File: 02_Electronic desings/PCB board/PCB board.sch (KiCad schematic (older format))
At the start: 26 parts, among them J1 M1 Encoder, J10 Switch Manual/Auto, J11 Jetson, J12 Compass, J14 Arduino_Header, J15 M2_Controll, J16 Power +5V, J17 GPS, J18 Power +5V, J19 Power +5V, J2 M2 Encoder, J20 I2C, J21 Power +5V, J22 XBee, J3 Power +5V, J4 M1 encoder, J5 PS2_Controll, J6 M2 encoder, J8 Arduino_Mega_Header, J9 M1_Controll, M1 Hercules_motordriver, M2 Hercules_motordriver, U1 PS2_Receiver, U2 BNO055, U3 Logic_Level_Converter, U4 Screw_term_p2_5mm

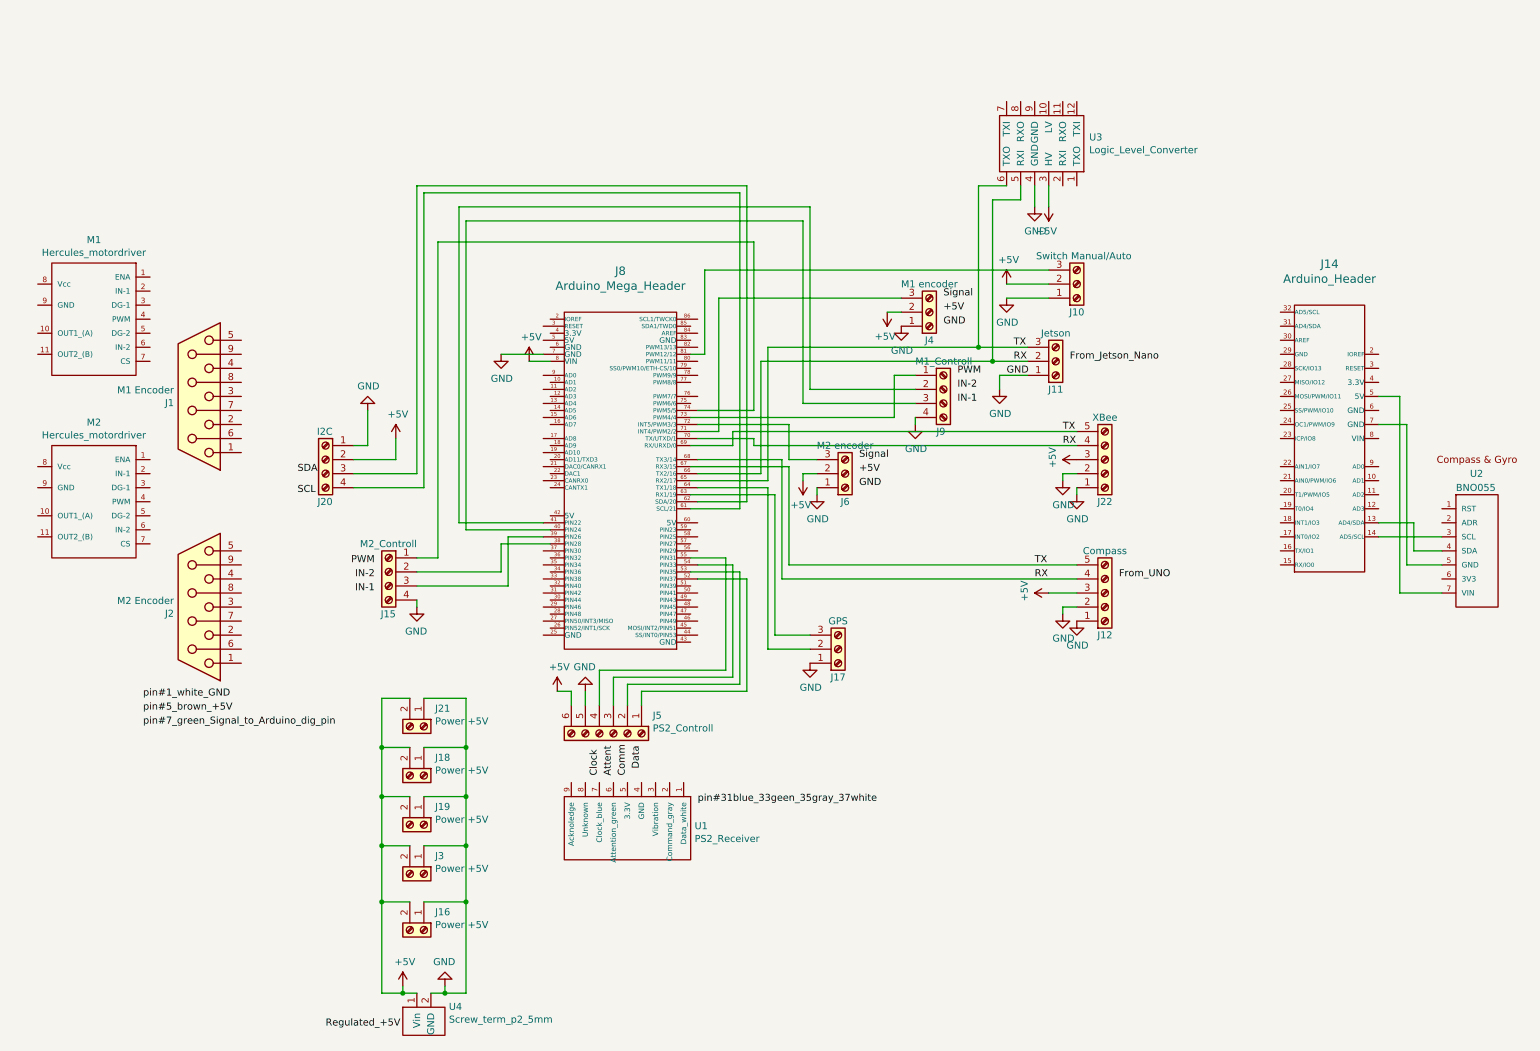
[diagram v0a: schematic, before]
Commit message: Upade
new version
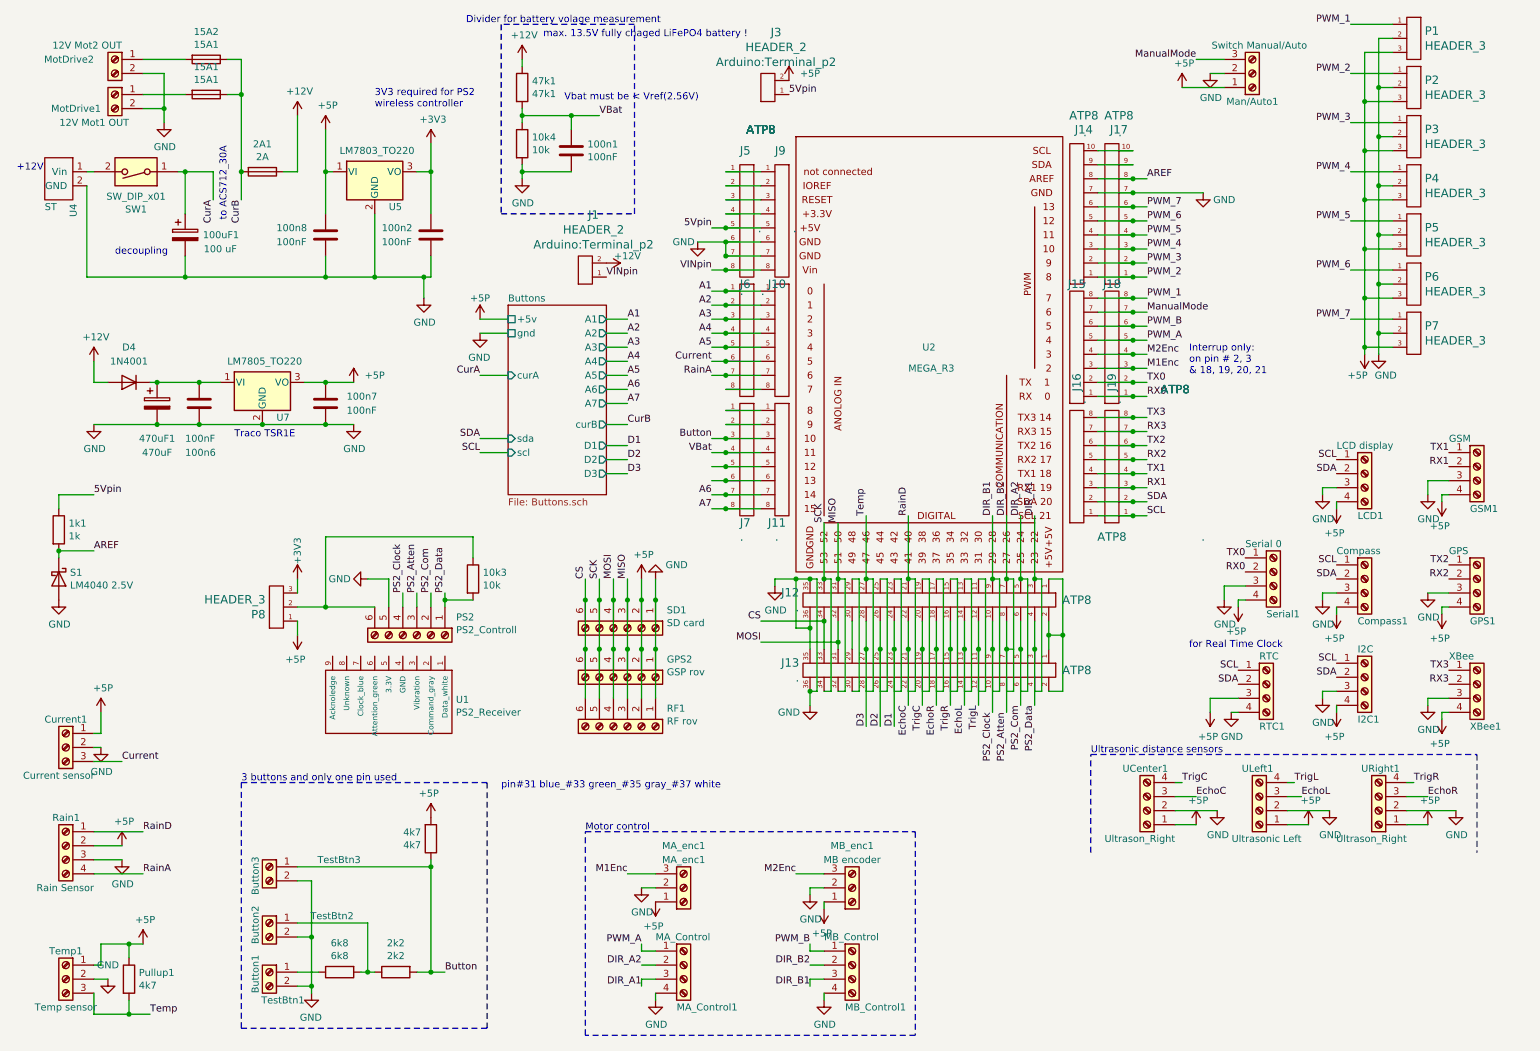
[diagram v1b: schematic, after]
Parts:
- removed J1: M1 Encoder, symbol Connector:DB9_Female
- removed J11: Jetson, TerminalBlock_TE-Connectivity:TerminalBlock_TE_282834-3_1x03_P2.54mm_Horizontal, symbol Connector:Screw_Terminal_01x03
- removed J12: Compass, TerminalBlock_TE-Connectivity:TerminalBlock_TE_282834-5_1x05_P2.54mm_Horizontal, symbol Connector:Screw_Terminal_01x05
- removed J14: Arduino_Header, symbol w_connectors:Arduino_Header
- removed J15: M2_Controll, TerminalBlock_TE-Connectivity:TerminalBlock_TE_282834-4_1x04_P2.54mm_Horizontal, symbol Connector:Screw_Terminal_01x04
- removed J16, J18, J19, J21, J3: Power +5V, TerminalBlock_TE-Connectivity:TerminalBlock_TE_282834-2_1x02_P2.54mm_Horizontal, symbol Connector:Screw_Terminal_01x02
- removed J17: GPS, TerminalBlock_TE-Connectivity:TerminalBlock_TE_282834-3_1x03_P2.54mm_Horizontal, symbol Connector:Screw_Terminal_01x03
- removed J2: M2 Encoder, symbol Connector:DB9_Female
- removed J20: I2C, TerminalBlock_TE-Connectivity:TerminalBlock_TE_282834-4_1x04_P2.54mm_Horizontal, symbol Connector:Screw_Terminal_01x04
- removed J22: XBee, TerminalBlock_TE-Connectivity:TerminalBlock_TE_282834-5_1x05_P2.54mm_Horizontal, symbol Connector:Screw_Terminal_01x05
- removed J8: Arduino_Mega_Header, Arduino:Arduino_MEGA, symbol w_connectors:Arduino_Mega_Header
- removed M1, M2: Hercules_motordriver, symbol My_symbol_library:Hercules_motordriver
- removed U2: BNO055, symbol My_symbol_library:BNO055
- removed U3: Logic_Level_Converter, Arduino:Logic_Level_Converter, symbol My_symbol_library:Logic_Level_Converter
- added 100n1, 100n2, 100n6, 100n7, 100n8: 100nF, Capacitor_THT:C_Disc_D10.5mm_W5.0mm_P5.00mm, symbol Device:C
- added 100uF1: 100 uF, Capacitor_THT:C_Radial_D8.0mm_H7.0mm_P3.50mm, symbol Device:CP
- added 10k3: 10k, Resistor_THT:R_Axial_DIN0207_L6.3mm_D2.5mm_P10.16mm_Horizontal, symbol Device:R
- added 10k4: 10k, Resistor_THT:R_Axial_DIN0309_L9.0mm_D3.2mm_P5.08mm_Vertical, symbol Device:R
- added 15A1, 15A2: 15A1, Shield:Fuse, symbol Device:Fuse
- added 1k1: 1k, Resistor_THT:R_Axial_DIN0207_L6.3mm_D2.5mm_P10.16mm_Horizontal, symbol Device:R
- added 2A1: 2A, Shield:Fuse, symbol Device:Fuse
- added 2k2: 2k2, Resistor_THT:R_Axial_DIN0309_L9.0mm_D3.2mm_P5.08mm_Vertical, symbol Device:R
- added 470uF1: 470uF, Capacitor_THT:C_Radial_D8.0mm_H7.0mm_P3.50mm, symbol Device:CP
- added 47k1: 47k1, Resistor_THT:R_Axial_DIN0309_L9.0mm_D3.2mm_P12.70mm_Horizontal, symbol Device:R
- added 4k7: 4k7, Resistor_THT:R_Axial_DIN0309_L9.0mm_D3.2mm_P5.08mm_Vertical, symbol Device:R
- added 6k8: 6k8, Resistor_THT:R_Axial_DIN0309_L9.0mm_D3.2mm_P5.08mm_Vertical, symbol Device:R
- added Button1: TestBtn1, Connector_JST:JST_XH_B2B-XH-A_1x02_P2.50mm_Vertical, symbol Connector:Screw_Terminal_01x02
- added Button2: TestBtn2, Connector_JST:JST_XH_B2B-XH-A_1x02_P2.50mm_Vertical, symbol Connector:Screw_Terminal_01x02
- added Button3: TestBtn3, Connector_JST:JST_XH_B2B-XH-A_1x02_P2.50mm_Vertical, symbol Connector:Screw_Terminal_01x02
- added Compass1: Compass, Connector_JST:JST_XH_B4B-XH-A_1x04_P2.50mm_Vertical, symbol Connector:Screw_Terminal_01x04
- added Current1: Current sensor, Connector_JST:JST_XH_B3B-XH-A_1x03_P2.50mm_Vertical, symbol Connector:Screw_Terminal_01x03
- added D4: 1N4001, Diode_THT:D_5W_P5.08mm_Vertical_AnodeUp, symbol Simulation_SPICE:DIODE
- added GPS1: GPS, Connector_JST:JST_XH_B4B-XH-A_1x04_P2.50mm_Vertical, symbol Connector:Screw_Terminal_01x04
- added GPS2: GSP rov, Connector_JST:JST_XH_B6B-XH-A_1x06_P2.50mm_Vertical, symbol Connector:Screw_Terminal_01x06
- added GSM1: GSM, Connector_JST:JST_XH_B4B-XH-A_1x04_P2.50mm_Vertical, symbol Connector:Screw_Terminal_01x04
- added I2C1: I2C, Connector_JST:JST_XH_B4B-XH-A_1x04_P2.50mm_Vertical, symbol Connector:Screw_Terminal_01x04
- added J1, J3: HEADER_2, Arduino:Terminal_p2, symbol w_connectors:HEADER_2
- added J10, J11, J15, J18, J19, J5, J6, J7, J9: ., ATP8, symbol w_connectors:HEADER_8
- added J12, J13: ., ATP8, symbol w_connectors:HEADER_18x2
- added J14, J17: ., ATP8, symbol w_connectors:HEADER_10
- added J16: ., ., symbol w_connectors:HEADER_8
- added LCD1: LCD display, Connector_JST:JST_XH_B4B-XH-A_1x04_P2.50mm_Vertical, symbol Connector:Screw_Terminal_01x04
- added MB_Control1: MB_Control, Connector_JST:JST_XH_B4B-XH-A_1x04_P2.50mm_Vertical, symbol Connector:Screw_Terminal_01x04
- added MotDrive1: 12V Mot1 OUT, TerminalBlock_Phoenix:TerminalBlock_Phoenix_MKDS-1,5-2-5.08_1x02_P5.08mm_Horizontal, symbol Connector:Screw_Terminal_01x02
- added MotDrive2: 12V Mot2 OUT, TerminalBlock_Phoenix:TerminalBlock_Phoenix_MKDS-1,5-2-5.08_1x02_P5.08mm_Horizontal, symbol Connector:Screw_Terminal_01x02
- added P1, P2, P3, P4, P5, P6, P7: HEADER_3, Arduino:Terminal_p3_sp, symbol w_connectors:HEADER_3
- added P8: HEADER_3, Arduino:Terminal_p3, symbol w_connectors:HEADER_3
- added Pullup1: 4k7, Resistor_THT:R_Axial_DIN0207_L6.3mm_D2.5mm_P10.16mm_Horizontal, symbol Device:R
- added RF1: RF rov, Connector_JST:JST_XH_B6B-XH-A_1x06_P2.50mm_Vertical, symbol Connector:Screw_Terminal_01x06
- added RTC1: RTC, Connector_JST:JST_XH_B4B-XH-A_1x04_P2.50mm_Vertical, symbol Connector:Screw_Terminal_01x04
- added Rain1: Rain Sensor, Connector_JST:JST_XH_B4B-XH-A_1x04_P2.50mm_Vertical, symbol Connector:Screw_Terminal_01x04
- added S1: LM4040 2.5V, Arduino:TO-92, symbol Device:D_Schottky
- added SD1: SD card, Connector_JST:JST_XH_B6B-XH-A_1x06_P2.50mm_Vertical, symbol Connector:Screw_Terminal_01x06
- added SW1: SW_DIP_x01, TerminalBlock_Phoenix:TerminalBlock_Phoenix_MKDS-1,5-2-5.08_1x02_P5.08mm_Horizontal, symbol Switch:SW_DIP_x01
- added Serial1: Serial 0, Connector_JST:JST_XH_B4B-XH-A_1x04_P2.50mm_Vertical, symbol Connector:Screw_Terminal_01x04
- added Temp1: Temp sensor, Connector_JST:JST_XH_B3B-XH-A_1x03_P2.50mm_Vertical, symbol Connector:Screw_Terminal_01x03
- added U2: MEGA_R3, symbol My_symbol_library:MEGA_R3
- added U5: LM7803_TO220, Package_TO_SOT_THT:TO-220-3_Vertical, symbol Regulator_Linear:LM7805_TO220
- added U7: LM7805_TO220, My_footprint_library:Traco_TSR2, symbol Regulator_Linear:LM7805_TO220
- added UCenter1, URight1: Ultrason_Right, Connector_JST:JST_XH_B4B-XH-A_1x04_P2.50mm_Vertical, symbol Connector:Screw_Terminal_01x04
- added ULeft1: Ultrasonic Left, Connector_JST:JST_XH_B4B-XH-A_1x04_P2.50mm_Vertical, symbol Connector:Screw_Terminal_01x04
- added XBee1: XBee, Connector_JST:JST_XH_B4B-XH-A_1x04_P2.50mm_Vertical, symbol Connector:Screw_Terminal_01x04
- MA_Control1: renamed from J9; value M1_Controll -> MA_Control; footprint TerminalBlock_TE-Connectivity:TerminalBlock_TE_282834-4_1x04_P2.54mm_Horizontal -> Connector_JST:JST_XH_B4B-XH-A_1x04_P2.50mm_Vertical
- MA_enc1: renamed from J4; value M1 encoder -> MA_enc1; footprint TerminalBlock_TE-Connectivity:TerminalBlock_TE_282834-3_1x03_P2.54mm_Horizontal -> Connector_JST:JST_XH_B3B-XH-A_1x03_P2.50mm_Vertical
- MB_enc1: renamed from J6; value M2 encoder -> MB encoder; footprint TerminalBlock_TE-Connectivity:TerminalBlock_TE_282834-3_1x03_P2.54mm_Horizontal -> Connector_JST:JST_XH_B3B-XH-A_1x03_P2.50mm_Vertical
- Man/Auto1: renamed from J10; footprint TerminalBlock_TE-Connectivity:TerminalBlock_TE_282834-3_1x03_P2.54mm_Horizontal -> Connector_JST:JST_XH_B3B-XH-A_1x03_P2.50mm_Vertical
- PS2: renamed from J5; footprint TerminalBlock_TE-Connectivity:TerminalBlock_TE_282834-6_1x06_P2.54mm_Horizontal -> Connector_JST:JST_XH_B6B-XH-A_1x06_P2.50mm_Vertical
- U4: value Screw_term_p2_5mm -> ST; footprint Arduino:Screw_term_p2_5mm -> TerminalBlock_Phoenix:TerminalBlock_Phoenix_MKDS-1,5-2-5.08_1x02_P5.08mm_Horizontal
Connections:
- net GND: now also MA_enc1.2 (Pin_2), MB_enc1.2 (Pin_2), Man/Auto1.2 (Pin_2), 100n1.2, 100n2.2, 100n6.2, 100n7.2, 100n8.2, 100uF1.2, 10k4.2, 470uF1.2, Button1.2 (Pin_2), Button2.2 (Pin_2), Button3.2 (Pin_2), Compass1.3 (Pin_3), Current1.2 (Pin_2), GPS1.3 (Pin_3), GPS2.1 (Pin_1), GSM1.3 (Pin_3), I2C1.3 (Pin_3), J12.35, J12.36, J13.35, J13.36, J14.7, J17.7, J5.6, J5.7, J9.6, J9.7, LCD1.3 (Pin_3), MB_Control1.4 (Pin_4), MotDrive1.2 (Pin_2), MotDrive2.2 (Pin_2), P1.2, P2.2, P3.2, P4.2, P5.2, P6.2, P7.2, RF1.1 (Pin_1), RTC1.4 (Pin_4), Rain1.3 (Pin_3), S1.2 (A), SD1.1 (Pin_1), Serial1.3 (Pin_3), Temp1.2 (Pin_2), U5.2 (GND), U7.2 (GND), UCenter1.2 (Pin_2), ULeft1.2 (Pin_2), URight1.2 (Pin_2), XBee1.3 (Pin_3); no longer MA_enc1.1 (Pin_1), MB_enc1.1 (Pin_1), Man/Auto1.1 (Pin_1)
- net SCL: now also Compass1.1 (Pin_1), I2C1.1 (Pin_1), J16.1, J19.1, LCD1.1 (Pin_1), RTC1.1 (Pin_1)
- net SDA: now also Compass1.2 (Pin_2), I2C1.2 (Pin_2), J16.2, J19.2, LCD1.2 (Pin_2), RTC1.2 (Pin_2)
- net DIR_A1: now reaches MA_Control1.3 (Pin_3)
- net DIR_A1: now also J12.3, J13.4
- net DIR_A2: now reaches MA_Control1.2 (Pin_2)
- net DIR_A2: now also J12.5, J13.6
- net PS2_Data: now reaches PS2.1 (Pin_1)
- net PS2_Data: now also 10k3.2, J12.4, J13.3
- net PS2_Com: now reaches PS2.2 (Pin_2)
- net PS2_Com: now also J12.6, J13.5
- net PS2_Atten: now reaches PS2.3 (Pin_3)
- net PS2_Atten: now also J12.8, J13.7
- net PS2_Clock: now reaches PS2.4 (Pin_4)
- net PS2_Clock: now also J12.10, J13.9
- net M1Enc: now reaches MA_enc1.3 (Pin_3)
- net M1Enc: now also J15.3, J18.3
- net M2Enc: now reaches MB_enc1.3 (Pin_3)
- net M2Enc: now also J15.4, J18.4
- net PWM_A: now reaches MA_Control1.1 (Pin_1)
- net PWM_A: now also J15.5, J18.5
- net ManualMode: now reaches Man/Auto1.3 (Pin_3)
- net ManualMode: now also J15.7, J18.7
- removed net +5V: MA_enc1.2 (Pin_2), MB_enc1.2 (Pin_2), Man/Auto1.2 (Pin_2), PS2.6 (Pin_6), U4.1 (Vin)
- new net: 10k3.1, P8.2, PS2.6 (Pin_6)
- new net: SW1.2, U4.1 (Vin)
- new net: 6k8.1, Button1.1 (Pin_1)
- new net: 2k2.1, 6k8.2, Button2.1 (Pin_1)
- new net: 15A1.2, MotDrive1.1 (Pin_1)
- new net: 15A2.2, MotDrive2.1 (Pin_1)
- new net: 100n6.1, 470uF1.1, D4.2 (K), U7.1 (VI)
- new net: J14.10, J17.10
- new net: J14.9, J17.9
- new net: J10.8, J6.8
- new net: J5.1, J9.1
- new net: J5.2, J9.2
- new net: J5.3, J9.3
- new net: J5.4, J9.4
- new net: J11.1, J7.1
- new net: J11.2, J7.2
- new net: J11.5, J7.5
- new net: J11.6, J7.6
- new net: J12.1, J12.2, J13.1, J13.2
- new net: J12.11, J13.12
- new net: J12.13, J13.14
- new net: J12.15, J13.16
- new net: J12.17, J13.18
- new net: J12.19, J13.20
- new net: J12.23, J13.24
- new net: J12.25, J13.26
- new net: J12.29, J13.30
- new net: J12.30, J13.29
- new net +12V: 2A1.1, 47k1.1, D4.1 (A), J1.2
- new net +3V3: 100n2.1, P8.3, U5.3 (VO)
- new net +5P: 100n7.1, 100n8.1, 4k7.2, Compass1.4 (Pin_4), Current1.1 (Pin_1), GPS1.4 (Pin_4), GPS2.2 (Pin_2), GSM1.4 (Pin_4), I2C1.4 (Pin_4), J3.2, LCD1.4 (Pin_4), MA_enc1.1 (Pin_1), MB_enc1.1 (Pin_1), Man/Auto1.1 (Pin_1), P1.3, P2.3, P3.3, P4.3, P5.3, P6.3, P7.3, P8.1, Pullup1.1, RF1.2 (Pin_2), RTC1.3 (Pin_3), Rain1.2 (Pin_2), SD1.2 (Pin_2), Serial1.4 (Pin_4), Temp1.1 (Pin_1), U5.1 (VI), U7.3 (VO), UCenter1.1 (Pin_1), ULeft1.1 (Pin_1), URight1.1 (Pin_1), XBee1.4 (Pin_4)
- new net 5Vpin: 1k1.1, J3.1, J5.5, J9.5
- new net A1: J10.1, J6.1
- new net A2: J10.2, J6.2
- new net A3: J10.3, J6.3
- new net A4: J10.4, J6.4
- new net A5: J10.5, J6.5
- new net A6: J11.7, J7.7
- new net A7: J11.8, J7.8
- new net AREF: 1k1.2, J14.8, J17.8, S1.1 (K)
- new net Button: 2k2.2, 4k7.1, Button3.1 (Pin_1), J11.3, J7.3
- new net CS: GPS2.6 (Pin_6), J12.34, J13.33, RF1.6 (Pin_6), SD1.6 (Pin_6)
- new net CurA: 100uF1.1, SW1.1
- new net CurB: 15A1.1, 15A2.1, 2A1.2
- new net Current: Current1.3 (Pin_3), J10.6, J6.6
- new net D1: J12.24, J13.23
- new net D2: J12.26, J13.25
- new net D3: J12.28, J13.27
- new net DIR_B1: J12.9, J13.10, MB_Control1.3 (Pin_3)
- new net DIR_B2: J12.7, J13.8, MB_Control1.2 (Pin_2)
- new net EchoC: J12.22, J13.21, UCenter1.3 (Pin_3)
- new net EchoL: J12.14, J13.13, ULeft1.3 (Pin_3)
- new net EchoR: J12.18, J13.17, URight1.3 (Pin_3)
- new net MISO: GPS2.3 (Pin_3), J12.31, J13.32, RF1.3 (Pin_3), SD1.3 (Pin_3)
- new net MOSI: GPS2.4 (Pin_4), J12.32, J13.31, RF1.4 (Pin_4), SD1.4 (Pin_4)
- new net PWM_1: J15.8, J18.8, P1.1
- new net PWM_2: J14.1, J17.1, P2.1
- new net PWM_3: J14.2, J17.2, P3.1
- new net PWM_4: J14.3, J17.3, P4.1
- new net PWM_5: J14.4, J17.4, P5.1
- new net PWM_6: J14.5, J17.5, P6.1
- new net PWM_7: J14.6, J17.6, P7.1
- new net PWM_B: J15.6, J18.6, MB_Control1.1 (Pin_1)
- new net RX0: J15.1, J18.1, Serial1.2 (Pin_2)
- new net RX1: GSM1.2 (Pin_2), J16.3, J19.3
- new net RX2: GPS1.2 (Pin_2), J16.5, J19.5
- new net RX3: J16.7, J19.7, XBee1.2 (Pin_2)
- new net RainA: J10.7, J6.7, Rain1.4 (Pin_4)
- new net RainD: J12.21, J13.22, Rain1.1 (Pin_1)
- new net SCK: GPS2.5 (Pin_5), J12.33, J13.34, RF1.5 (Pin_5), SD1.5 (Pin_5)
- new net TX0: J15.2, J18.2, Serial1.1 (Pin_1)
- new net TX1: GSM1.1 (Pin_1), J16.4, J19.4
- new net TX2: GPS1.1 (Pin_1), J16.6, J19.6
- new net TX3: J16.8, J19.8, XBee1.1 (Pin_1)
- new net Temp: J12.27, J13.28, Pullup1.2, Temp1.3 (Pin_3)
- new net TrigC: J12.20, J13.19, UCenter1.4 (Pin_4)
- new net TrigL: J12.12, J13.11, ULeft1.4 (Pin_4)
- new net TrigR: J12.16, J13.15, URight1.4 (Pin_4)
- new net VBat: 100n1.1, 10k4.1, 47k1.2, J11.4, J7.4
- new net VINpin: J1.1, J5.8, J9.8
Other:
- note added: "+12V"
- note added: "3 buttons and only one pin used"
- note added: "3V3 required for PS2\nwireless controller"
- note added: "Divider for battery volage measurement"
- note added: "Interrup only:\non pin # 2, 3\n& 18, 19, 20, 21"
- note added: "Motor control"
- note added: "Traco TSR1E"
- note added: "Ultrasonic distance sensors"
- note added: "Vbat must be < Vref(2.56V)"
- note added: "decoupling"
- note added: "for Real Time Clock"
- note added: "max. 13.5V fully chaged LiFePO4 battery !"
- note added: "pin#31 blue_#33 green_#35 gray_#37 white"
- note added: "to ACS712_30A"
- moved on the sheet: MA_Control1, MA_enc1, MB_enc1, Man/Auto1, PS2, U1, U4
